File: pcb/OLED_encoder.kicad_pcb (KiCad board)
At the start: 2 copper layers, 135 x 38 mm, 21 parts, among them J1 Conn_01x10, J2 Conn_02x08_Odd_Even, U1 ACZ11BR1E-20FD1-20C

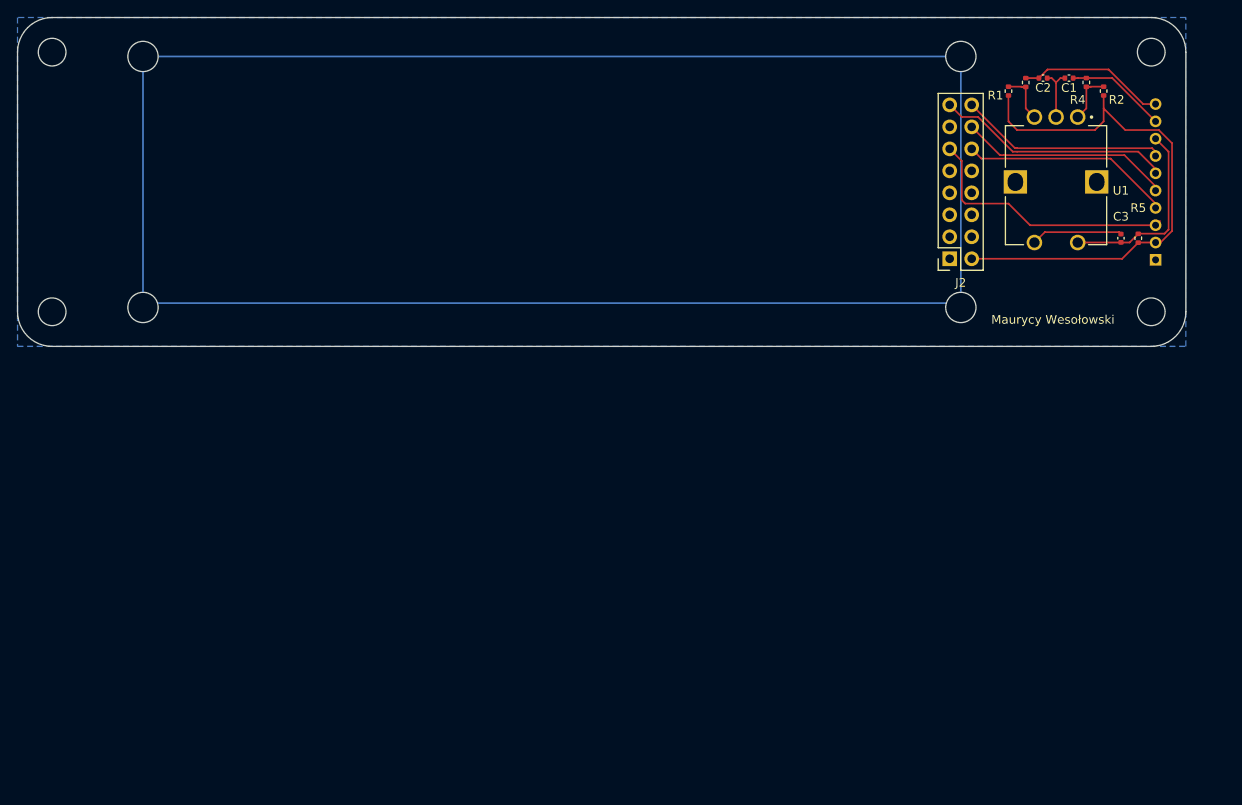
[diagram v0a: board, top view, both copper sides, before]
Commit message: refactor
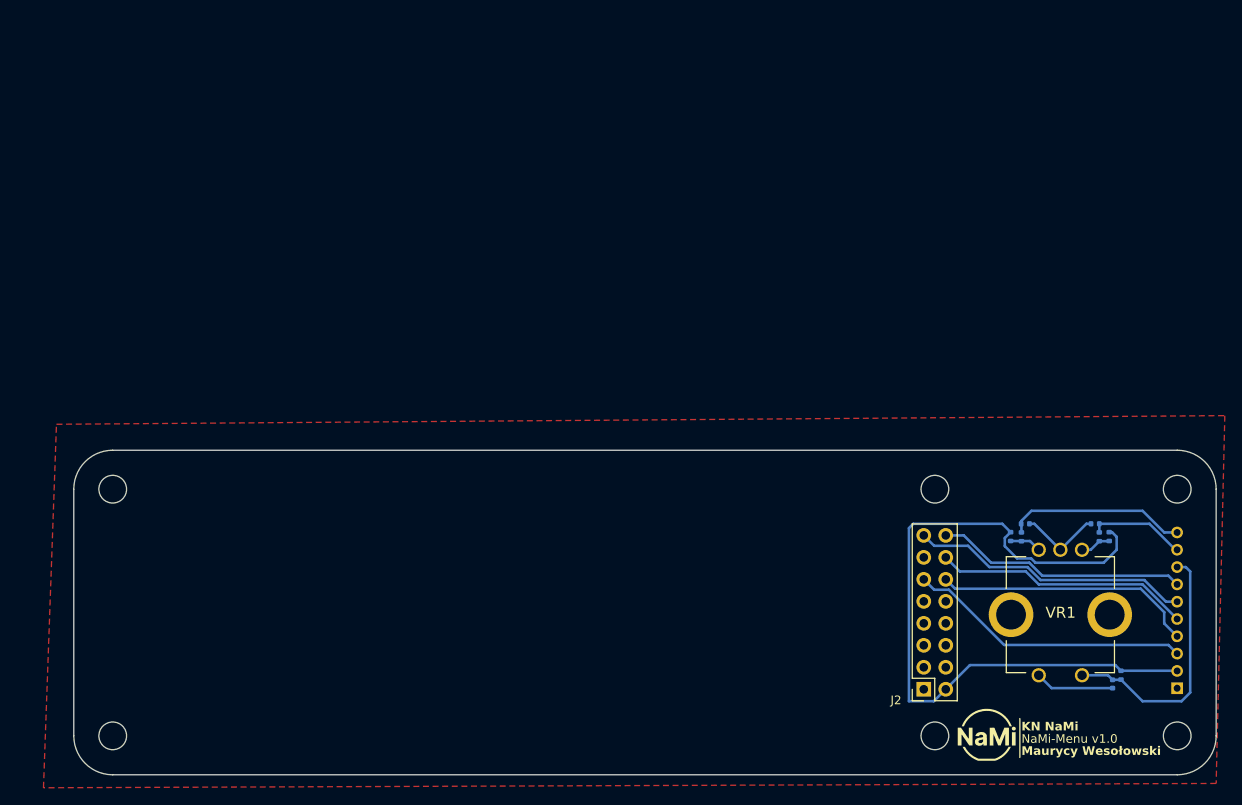
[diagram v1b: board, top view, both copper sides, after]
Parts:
- removed the G*** at (135.5, 77.0)
- removed the G*** at (129.5, 68.5)
- removed H7, H8: MountingHole, MountingHole:MountingHole_3.5mm
- removed U1: ACZ11BR1E-20FD1-20C, ACZ11BR1E-20FD1-20C:CUI_ACZ11BR1E-20FD1-20C
- added G***: LOGO, Symbol:NaMi-logo, F.Cu at (157.0, 132.9)
- added VR1: ENCODER, Library:PEC11R4220FS0024, F.Cu at (168.0, 126.0)
- C1, C2, C3, R1, R2, R3, R4, R5: moved to B.Cu
- H5, H6: footprint MountingHole:MountingHole_3.5mm -> MountingHole:MountingHole_3.2mm_M3
- moved H1 130.2 mm to (56.0, 104.5)
- moved H6 129.3 mm to (179.0, 133.0)
- moved H3 104.0 mm to (151.0, 104.5)
- moved H2 79.3 mm to (56.0, 133.0)
- moved H5 55.9 mm to (179.0, 104.5)
- moved H4 55.0 mm to (151.0, 133.0)
- moved R3 53.3 mm to (171.1, 110.0)
- moved R2 52.6 mm to (159.7, 110.0), turned to -90 degrees
- moved R4 52.5 mm to (170.0, 110.0), turned to -90 degrees
- moved C2 51.9 mm to (169.5, 108.5), turned to 180 degrees
- moved C1 51.7 mm to (161.4, 108.5), turned to 0 degrees
- moved R1 51.5 mm to (161.0, 110.0)
- moved C3 51.5 mm to (171.5, 127.0), turned to -90 degrees
- moved R5 50.5 mm to (172.5, 126.0), turned to -90 degrees
- moved J2 49.8 mm to (149.7, 127.6)
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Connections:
- C1 pad 1: SIG A OUT -> SIG B OUT
- C2 pad 1: SIG B OUT -> SIG A OUT
- R1 pad 1: VCC -> Net-(VR1-B)
- R1 pad 2: Net-(R1-Pad2) -> SIG B OUT
- R2 pad 2: Net-(R2-Pad2) -> Net-(VR1-B)
- R3 pad 1: SIG B OUT -> VCC
- R3 pad 2: Net-(R1-Pad2) -> Net-(VR1-A)
- R4 pad 1: Net-(R2-Pad2) -> SIG A OUT
- R4 pad 2: SIG A OUT -> Net-(VR1-A)
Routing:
- net VCC: track 62.0 -> 84.2 mm
- net S1: track 22.7 -> 29.9 mm
- net SCLK: track 24.6 -> 30.6 mm
- net Net-(R2-Pad2): track 5.93 -> 0.00 mm
- net Net-(R1-Pad2): track 5.91 -> 0.00 mm
- net DC: track 24.8 -> 29.7 mm
- net RESET: track 27.6 -> 32.4 mm
- net CS: track 24.2 -> 29.1 mm
- net Net-(VR1-B): track 0.00 -> 3.67 mm
- net Net-(VR1-A): track 0.00 -> 3.56 mm
- net SIG B OUT: track 17.3 -> 20.9 mm
- net MOSI: track 31.1 -> 32.8 mm
- net GND: track 17.1 -> 18.7 mm
- added copper zone on F.Cu, net GND
- removed copper zone on B.Cu, net GND
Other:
- board size 135 x 38 mm -> 132 x 37.5 mm
- board text added: "KN NaMi"
- board text added: "NaMi-Menu v1.0"
